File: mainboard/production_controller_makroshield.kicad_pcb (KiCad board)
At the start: 2 copper layers, 165.1 x 204 mm, 113 parts, among them J1 CON_TERM_BLK_1X2_TB008A-508-0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, J10 CON_CONNAXIO_MOTOR_DRIVER, J11 CON_CONNAXIO_MOTOR_DRIVER, J12 CON_CONNAXIO_MOTOR_DRIVER, J13 CON_CONNAXIO_MOTOR_DRIVER, J14 CON_CONNAXIO_MOTOR_DRIVER, J15 CON_CONNAXIO_MOTOR_DRIVER, J16 CON_CONNAXIO_MOTOR_DRIVER, J17 CON_CONNAXIO_MOTOR_DRIVER, J18 CON_CONNAXIO_MOTOR_DRIVER, J19 CON_CONNAXIO_MOTOR_DRIVER, J2 CON_TERM_BLK_1X2_TB008A-508-0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, J20 CON_CONNAXIO_MOTOR_DRIVER, J21 CON_CONNAXIO_MOTOR_DRIVER, J3 CON_HDR_MIKROBUS_ADDON_TH, J4 CON_TERM_BLK_1X2_TB008A-508-0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, J5 CON_HDR_MIKROBUS_SOCKET_TH, J6 CON_HDR_100MILS_M_TH_1X3, J7 CON_CONNAXIO_MOTOR_DRIVER, J8 CON_CONNAXIO_MOTOR_DRIVER, J9 CON_CONNAXIO_MOTOR_DRIVER, Q1 TRX_PMOS_AOD4189, Q2 TRX_2NPN_BC846S,115, U1 IO_EXP_PI4IOE5V6416ZDEX, U2 IO_EXP_PI4IOE5V6416ZDEX, U3 SEN_TEMP_TMP1075DR, U4 SEN_CUR_ACS711KEXLT-31AB-T, U5 ADC_NAU7802SGI

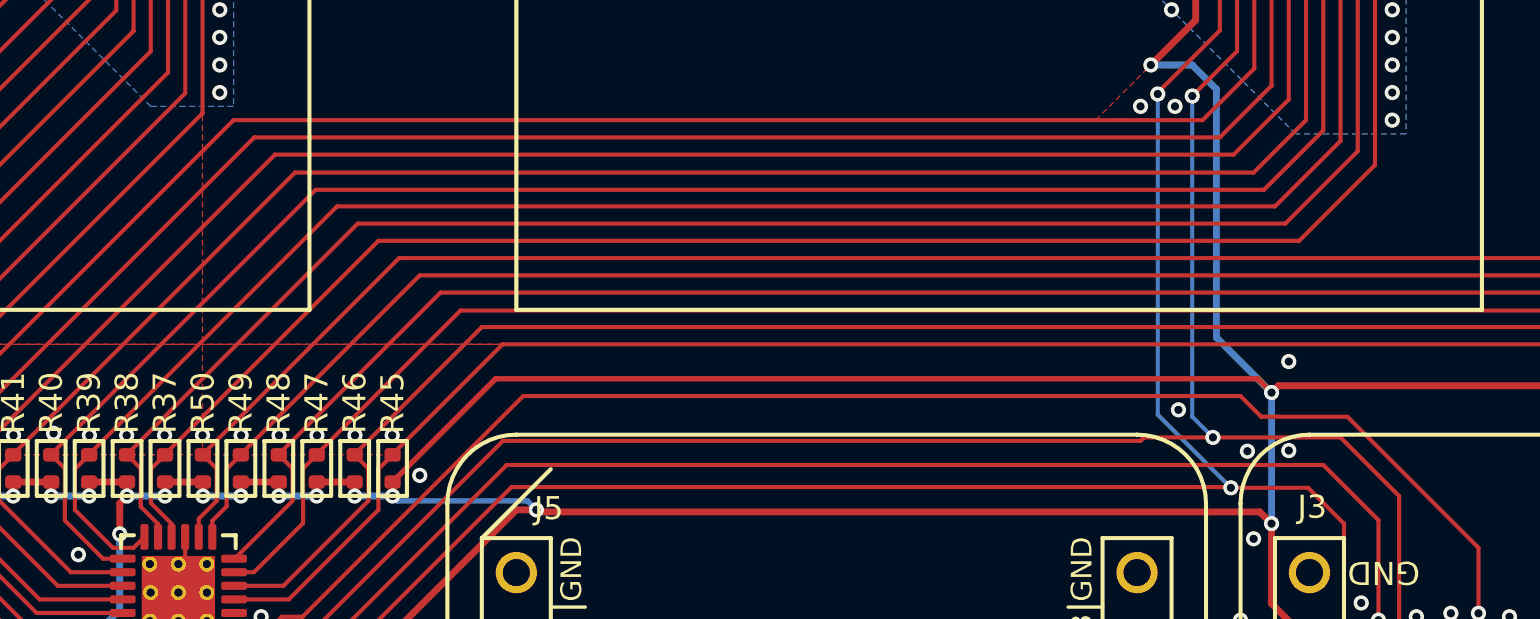
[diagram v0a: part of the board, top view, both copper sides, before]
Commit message: DRC pass
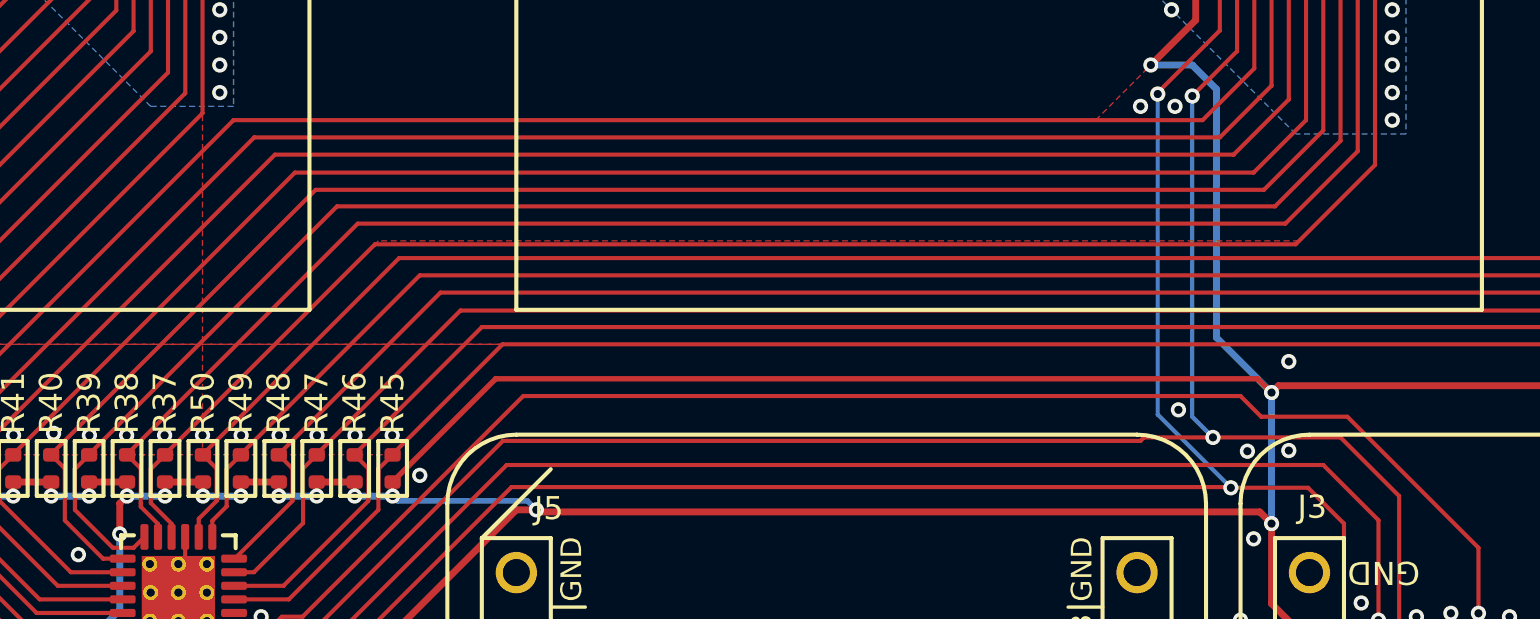
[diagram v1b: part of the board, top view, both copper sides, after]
